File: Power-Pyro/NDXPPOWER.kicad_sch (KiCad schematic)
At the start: 43 parts, among them J1 Conn_01x02, J5 Conn_01x02, J6 Conn_01x02, J7 Conn_01x02, Q1 SSM3J328R, Q2 SSM3J328R, Q3 L2N7002SLLT1G, Q4 L2N7002SLLT1G, Q5 SSM3J328R, Q6 SSM3J328R, Q7 L2N7002SLLT1G, Q8 L2N7002SLLT1G, U7 AP63203WU

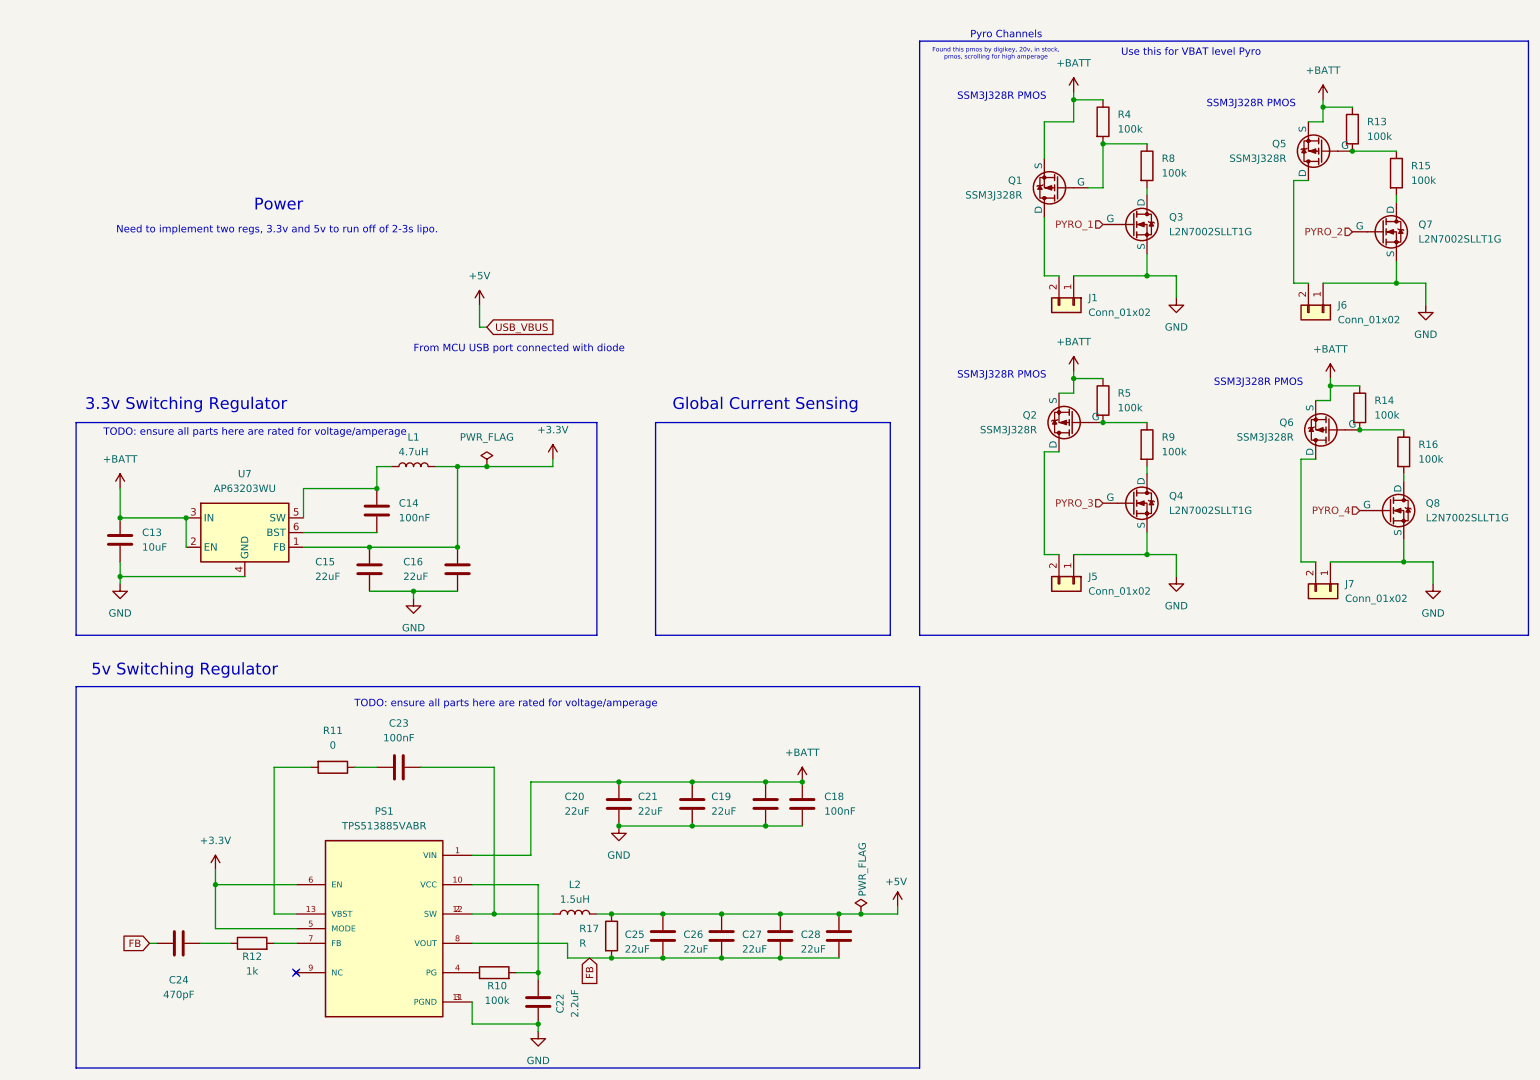
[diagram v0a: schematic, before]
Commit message: refactor🧮
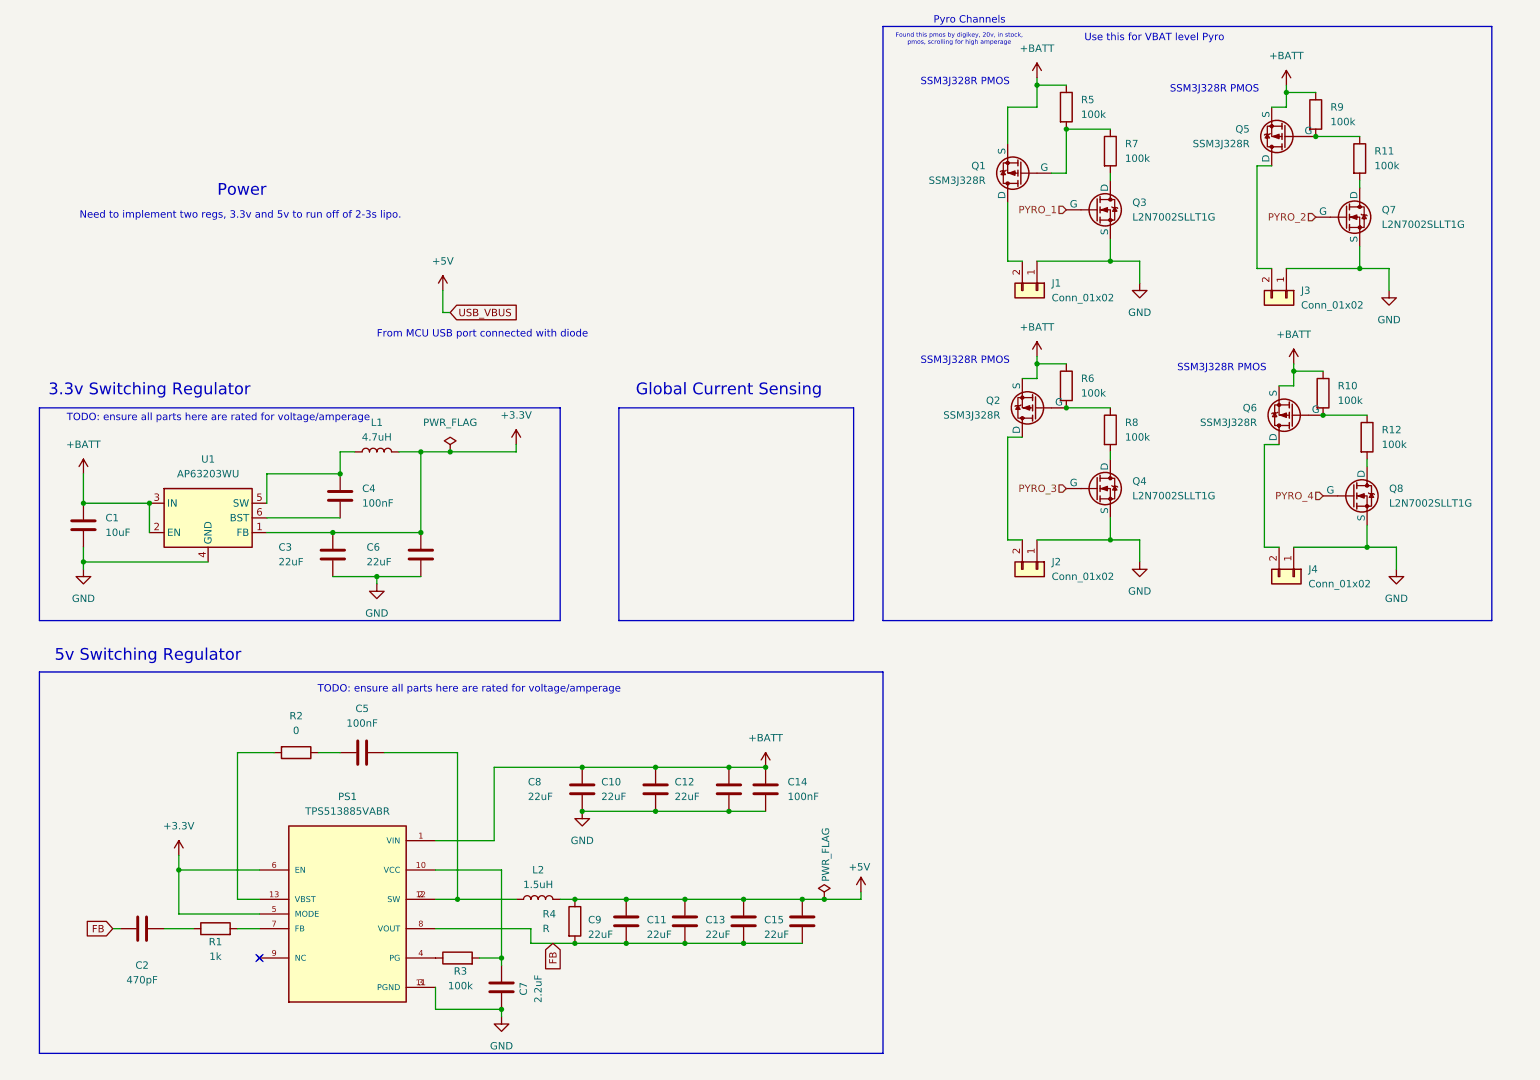
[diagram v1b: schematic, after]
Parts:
- removed C16, C19, C20, C21, C25, C26, C27, C28: 22uF, Capacitor_SMD:C_1206_3216Metric, symbol Device:C
- removed C18, C23: 100nF, Capacitor_SMD:C_0402_1005Metric, symbol Device:C
- removed C22: 2.2uF, Capacitor_SMD:C_0603_1608Metric, symbol Device:C
- removed C24: 470pF, Capacitor_SMD:C_0402_1005Metric, symbol Device:C
- removed J5, J6, J7: Conn_01x02, symbol Connector_Generic:Conn_01x02
- removed R13, R14, R15, R16: 100k, Resistor_SMD:R_0603_1608Metric, symbol Device:R
- removed R17: R, symbol Device:R
- removed U7: AP63203WU, Package_TO_SOT_SMD:TSOT-23-6, symbol Regulator_Switching:AP63203WU
- added C1: 10uF, Capacitor_SMD:C_0805_2012Metric, symbol Device:C
- added C10, C11, C12, C3, C6, C8, C9: 22uF, Capacitor_SMD:C_1206_3216Metric, symbol Device:C
- added C2: 470pF, Capacitor_SMD:C_0402_1005Metric, symbol Device:C
- added C4, C5: 100nF, Capacitor_SMD:C_0402_1005Metric, symbol Device:C
- added C7: 2.2uF, Capacitor_SMD:C_0603_1608Metric, symbol Device:C
- added J2, J3, J4: Conn_01x02, symbol Connector_Generic:Conn_01x02
- added R1: 1k, Resistor_SMD:R_0402_1005Metric, symbol Device:R
- added R2: 0, symbol Device:R
- added R3, R6, R7: 100k, Resistor_SMD:R_0603_1608Metric, symbol Device:R
- added U1: AP63203WU, Package_TO_SOT_SMD:TSOT-23-6, symbol Regulator_Switching:AP63203WU
- C13: value 10uF -> 22uF; footprint Capacitor_SMD:C_0805_2012Metric -> Capacitor_SMD:C_1206_3216Metric
- R11: value 0 -> 100k; footprint (none) -> Resistor_SMD:R_0603_1608Metric
- R12: value 1k -> 100k; footprint Resistor_SMD:R_0402_1005Metric -> Resistor_SMD:R_0603_1608Metric
- R4: value 100k -> R; footprint Resistor_SMD:R_0603_1608Metric -> (none)
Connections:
- net +3.3V: now also C3.1, C6.1, U1.1 (FB); no longer C15.1
- net +5V: now also C13.1, C15.1, R4.1, C11.1, C9.1
- net +BATT: now also C14.1, R10.1, R9.1, C1.1, C10.1, C12.1, C8.1, R6.1, U1.2 (EN), U1.3 (IN); no longer C13.1, R4.1
- net FB: now also C13.2, C15.2, R4.2, C11.2, C2.1, C9.2
- net GND: now also C14.2, C1.2, C10.2, C12.2, C3.2, C6.2, C7.1, C8.2, J2.1 (Pin_1), J3.1 (Pin_1), J4.1 (Pin_1), U1.4 (GND); no longer C13.2, C15.2
- net at L1.1: now also C4.1, U1.5 (SW); no longer C14.1
- net at Q8.1 (D): now also R12.2
- net at R9.2: now also Q5.2 (G), R11.1; no longer Q4.1 (D)
- net at Q6.1 (D): now also J4.2 (Pin_2)
- net at Q6.2 (G): now also R10.2, R12.1
- net at Q5.1 (D): now also J3.2 (Pin_2)
- net at PS1.10 (VCC): now also C7.2, R3.2; no longer R10.2
- net at L2.1, PS1.12 (SW), PS1.2 (SW): now also C5.2
- net at R11.2: now also Q7.1 (D); no longer PS1.13 (VBST)
- net at PS1.4 (PG): now also R3.1; no longer R10.1
- net at PS1.7 (FB): now also R1.2; no longer R12.2
- net at Q2.1 (D): now also J2.2 (Pin_2)
- net at Q3.1 (D): now also R7.2; no longer R8.2
- new net: C4.2, U1.6 (BST)
- new net: Q1.2 (G), R5.2, R7.1
- new net: PS1.13 (VBST), R2.2
- new net: Q2.2 (G), R6.2, R8.1
- new net: C2.2, R1.1
- new net: C5.1, R2.1
- new net: Q4.1 (D), R8.2
